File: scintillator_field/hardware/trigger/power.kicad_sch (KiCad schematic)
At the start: 18 parts, among them U1 LT3461A, U2 TPS7A4701, U3 TPS7A4701

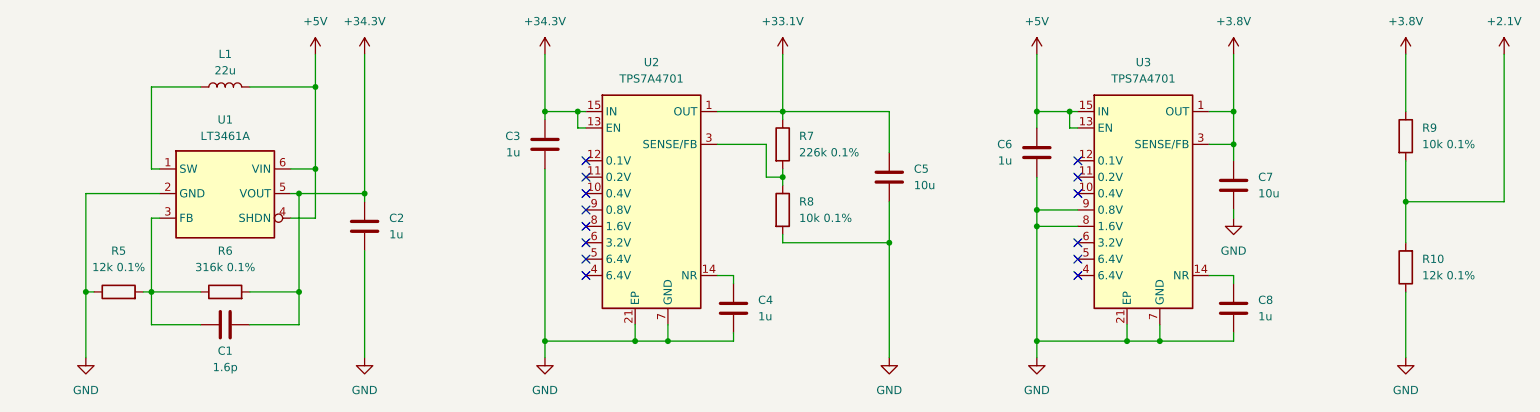
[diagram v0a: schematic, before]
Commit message: pcb v1
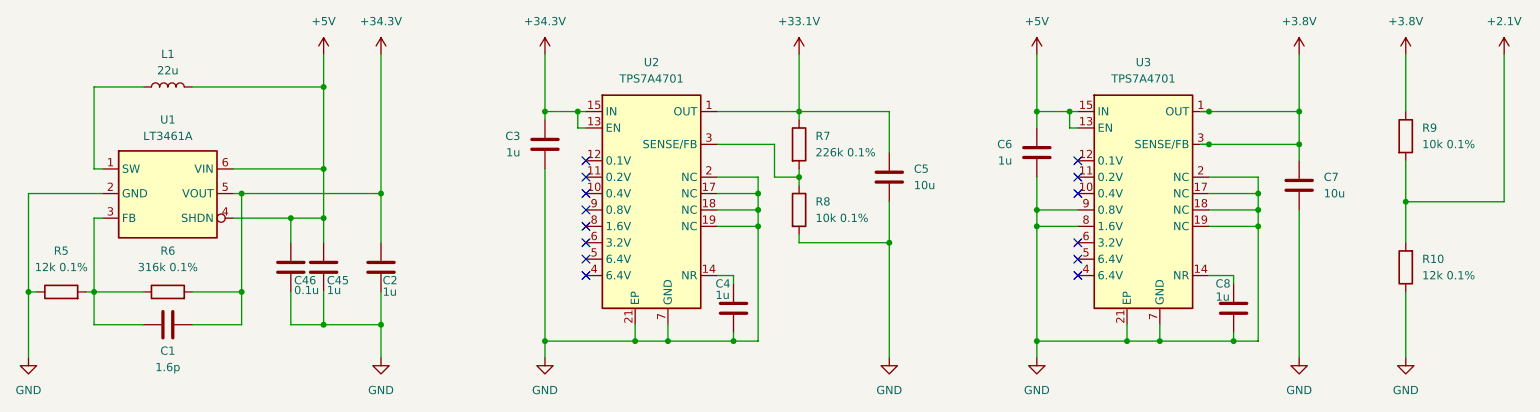
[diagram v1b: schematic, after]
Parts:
- added C45: 1u, Capacitor_SMD:C_0402_1005Metric, symbol Device:C
- added C46: 0.1u, Capacitor_SMD:C_0402_1005Metric, symbol Device:C
- L1: footprint (none) -> lqh3npn:L_Murata_LQH3NPN_3.0x3.0mm
- R10, R5: footprint (none) -> Resistor_SMD:R_0402_1005Metric
- R6, R7, R8, R9: footprint (none) -> Resistor_SMD:R_0603_1608Metric
- U2, U3: symbol Regulator_Linear:TPS7A4701xRGW -> tps7a4701:TPS7A4701xRGW
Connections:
- net +5V: now also C45.1, C46.1
- net GND: now also U2.17 (NC), U2.18 (NC), U2.19 (NC), U2.2 (NC), U3.17 (NC), U3.18 (NC), U3.19 (NC), U3.2 (NC), C45.2, C46.2
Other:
- moved on the sheet: C1, C2, C7, L1, R5, R6, R7, R8, U1

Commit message: pcb fabrication files
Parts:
- C1: LCSC (none) -> C88923
- C2, C3, C4, C45, C6, C8: LCSC (none) -> C52923
- C46: LCSC (none) -> C1581
- C5, C7: LCSC (none) -> C13585
- L1: LCSC (none) -> C237408
- R10, R5: LCSC (none) -> C317927
- R6: LCSC (none) -> C861317
- R7: LCSC (none) -> C861233
- R8, R9: LCSC (none) -> C136139
- U1: LCSC (none) -> C481768
- U2, U3: LCSC (none) -> C90084
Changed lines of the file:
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@@
+			)
+		)
+		(property "LCSC" "C136139"
+			(at 149.86 99.06 0)
+			(effects
+				(font
+					(size 1.27 1.27)
+				)
+				(hide yes)
 			)
 		)
@@
 			)
 		)
+		(property "LCSC" "C88923"
+			(at 52.07 116.84 0)
+			(effects
+				(font
+					(size 1.27 1.27)
+				)
+				(hide yes)
+			)
+		)
 		(pin "2"
 		)
@@
 			)
 		)
+		(property "LCSC" "C481768"
+			(at 52.07 96.52 0)
+			(effects
+				(font
+					(size 1.27 1.27)
+				)
+				(hide yes)
+			)
+		)
 		(pin "1"
 		)
@@
 			)
 		)
+		(property "LCSC" "C317927"
+			(at 35.56 111.76 0)
+			(effects
+				(font
+					(size 1.27 1.27)
+				)
+				(hide yes)
+			)
+		)
 		(pin "2"
 		)
@@
 			)
 		)
+		(property "LCSC" "C52923"
+			(at 217.17 114.3 0)
+			(effects
+				(font
+					(size 1.27 1.27)
+				)
+				(hide yes)
+			)
+		)
 		(pin "2"
 		)
@@
 			)
 		)
+		(property "LCSC" "C317927"
+			(at 243.84 107.95 0)
+			(effects
+				(font
+					(size 1.27 1.27)
+				)
+				(hide yes)
+			)
+		)
 		(pin "2"
 		)
@@
 			)
 		)
+		(property "LCSC" "C237408"
+			(at 52.07 80.01 0)
+			(effects
+				(font
+					(size 1.27 1.27)
+				)
+				(hide yes)
+			)
+		)
 		(pin "1"
 		)
@@
 			)
 		)
+		(property "LCSC" "C1581"
+			(at 71.12 107.95 0)
+			(effects
+				(font
+					(size 1.27 1.27)
+				)
+				(hide yes)
+			)
+		)
 		(pin "2"
 		)
@@
 		)
 		(property "Description" "Unpolarized capacitor"
+			(at 76.2 107.95 0)
+			(effects
+				(font
+					(size 1.27 1.27)
+				)
+				(hide yes)
+			)
+		)
+		(property "LCSC" "C52923"
 			(at 76.2 107.95 0)
 			(effects
@@
 			)
 		)
+		(property "LCSC" "C52923"
+			(at 110.49 88.9 0)
+			(effects
+				(font
+					(size 1.27 1.27)
+				)
+				(hide yes)
+			)
+		)
 		(pin "2"
 		)
@@
 			)
 		)
+		(property "LCSC" "C90084"
+			(at 203.2 99.06 0)
+			(effects
+				(font
+					(size 1.27 1.27)
+				)
+				(hide yes)
+			)
+		)
 		(pin "5"
 		)
@@
 			)
 		)
+		(property "LCSC" "C136139"
+			(at 243.84 87.63 0)
+			(effects
+				(font
+					(size 1.27 1.27)
+				)
+				(hide yes)
+			)
+		)
 		(pin "1"
 		)
@@
 		)
 		(property "Description" "Unpolarized capacitor"
+			(at 139.7 114.3 0)
+			(effects
+				(font
+					(size 1.27 1.27)
+				)
+				(hide yes)
+			)
+		)
+		(property "LCSC" "C52923"
 			(at 139.7 114.3 0)
 			(effects
@@
 			)
 		)
+		(property "LCSC" "C52923"
+			(at 186.69 90.17 0)
+			(effects
+				(font
+					(size 1.27 1.27)
+				)
+				(hide yes)
+			)
+		)
 		(pin "2"
 		)
@@
 			)
 		)
+		(property "LCSC" "C13585"
+			(at 163.83 93.98 0)
+			(effects
+				(font
+					(size 1.27 1.27)
+				)
+				(hide yes)
+			)
+		)
 		(pin "1"
 		)
@@
 			)
 		)
+		(property "LCSC" "C52923"
+			(at 85.09 107.95 0)
+			(effects
+				(font
+					(size 1.27 1.27)
+				)
+				(hide yes)
+			)
+		)
 		(pin "2"
 		)
@@
 			)
 		)
+		(property "LCSC" "C861317"
+			(at 52.07 111.76 0)
+			(effects
+				(font
+					(size 1.27 1.27)
+				)
+				(hide yes)
+			)
+		)
 		(pin "1"
 		)
@@
 			)
 		)
+		(property "LCSC" "C90084"
+			(at 127 99.06 0)
+			(effects
+				(font
+					(size 1.27 1.27)
+				)
+				(hide yes)
+			)
+		)
 		(pin "5"
 		)
@@
 			)
 		)
+		(property "LCSC" "C861233"
+			(at 149.86 88.9 0)
+			(effects
+				(font
+					(size 1.27 1.27)
+				)
+				(hide yes)
+			)
+		)
 		(pin "1"
 		)
@@
 			(at 227.33 95.25 0)
 			(effects
+				(font
+					(size 1.27 1.27)
+				)
+				(hide yes)
+			)
+		)
+		(property "LCSC" "C13585"
+			(at 227.33 95.25 0)
+			(effects
